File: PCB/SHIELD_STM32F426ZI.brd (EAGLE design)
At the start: 92.4 x 119.5 mm, 16 parts, among them IC1 AS4C16M16SA-6TCN, J1 104239-1430

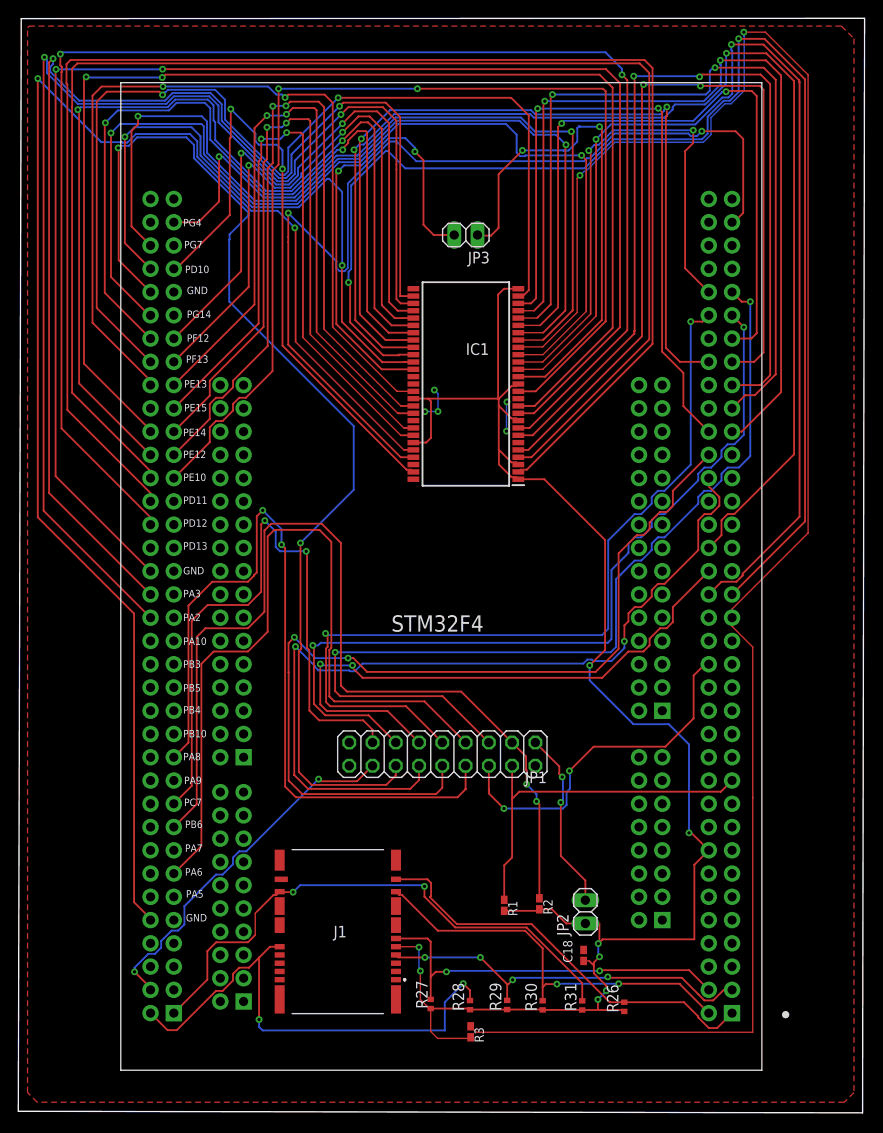
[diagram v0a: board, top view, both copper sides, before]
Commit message: PCB wurde mit kurzer Leitung korrigiert
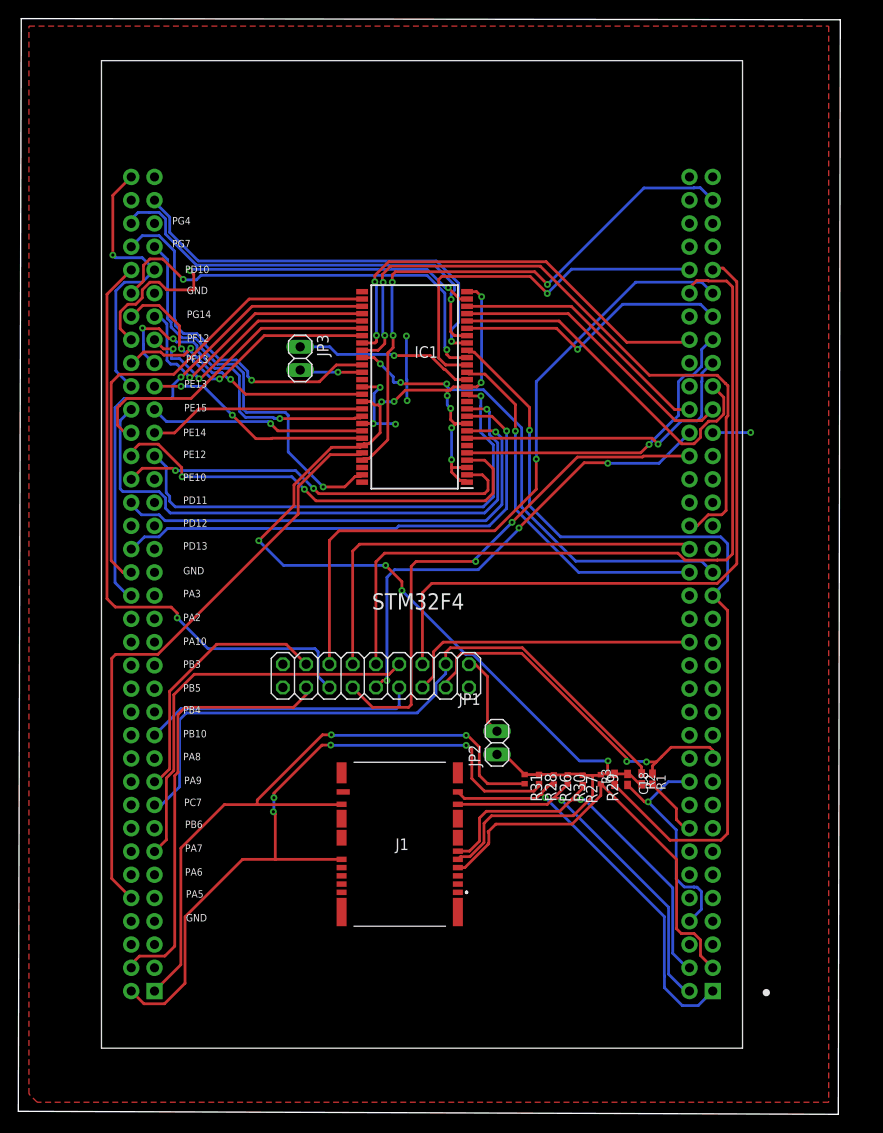
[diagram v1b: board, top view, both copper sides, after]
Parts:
- moved R3 31.7 mm to (65.9, 36.3), turned to 90 degrees
- moved R27 29.6 mm to (62.4, 36.2), turned to 270 degrees
- moved R29 26.7 mm to (64.4, 36.3), turned to 270 degrees
- moved R26 26.0 mm to (59.3, 36.3), turned to 270 degrees
- moved R28 25.8 mm to (57.7, 36.4), turned to 270 degrees
- moved R31 25.5 mm to (56.1, 36.3), turned to 270 degrees
- moved R30 24.8 mm to (60.8, 36.3), turned to 270 degrees
- moved JP3 22.6 mm to (31.6, 82.3), turned to 270 degrees
- moved R1 21.3 mm to (70.0, 36.3)
- moved JP2 20.8 mm to (53.1, 40.3)
- moved C18 19.8 mm to (67.3, 36.3), turned to 270 degrees
- moved R2 17.6 mm to (68.9, 36.4)
- moved J1 11.7 mm to (42.5, 20.3)
- moved JP1 11.2 mm to (39.9, 47.6)
- moved IC1 5.61 mm to (44.1, 79.2)
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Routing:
- net FMC_D0: track 166.7 -> 44.4 mm, vias 0 -> 2
- net FMC_D1: track 160.7 -> 49.7 mm, vias 0 -> 2
- net FMC_SDNE0: track 201.3 -> 91.6 mm, vias 2 -> 1
- net FMC_D4: track 162.8 -> 53.6 mm, vias 2 -> 1
- net FMC_D5: track 163.0 -> 56.3 mm, vias 2 -> 1
- net FMC_D13: track 163.8 -> 65.4 mm, vias 2 -> 0
- net FMC_SDCKE0: track 147.3 -> 53.5 mm, vias 2 -> 3
- net FMC_A5: track 139.1 -> 53.8 mm, vias 2 -> 1
- net FMC_SDNWE: track 122.8 -> 40.0 mm, vias 2 -> 1
- net FMC_A4: track 135.8 -> 53.3 mm, vias 2 -> 0
- net FMC_D6: track 140.1 -> 65.3 mm, vias 2 -> 1
- net FMC_A8: track 108.1 -> 34.1 mm, vias 2 -> 0
- net GND: track 7.15 -> 77.8 mm, vias 5 -> 8
- net FMC_D8: track 98.1 -> 28.5 mm
- net FMC_D7: track 121.8 -> 54.9 mm, vias 2 -> 1
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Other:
- board size 92.4 x 119.5 mm -> 89.8 x 119.7 mm
